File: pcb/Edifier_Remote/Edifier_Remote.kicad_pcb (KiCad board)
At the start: 2 copper layers, 4 parts, among them Q1 Q_NPN_BCE

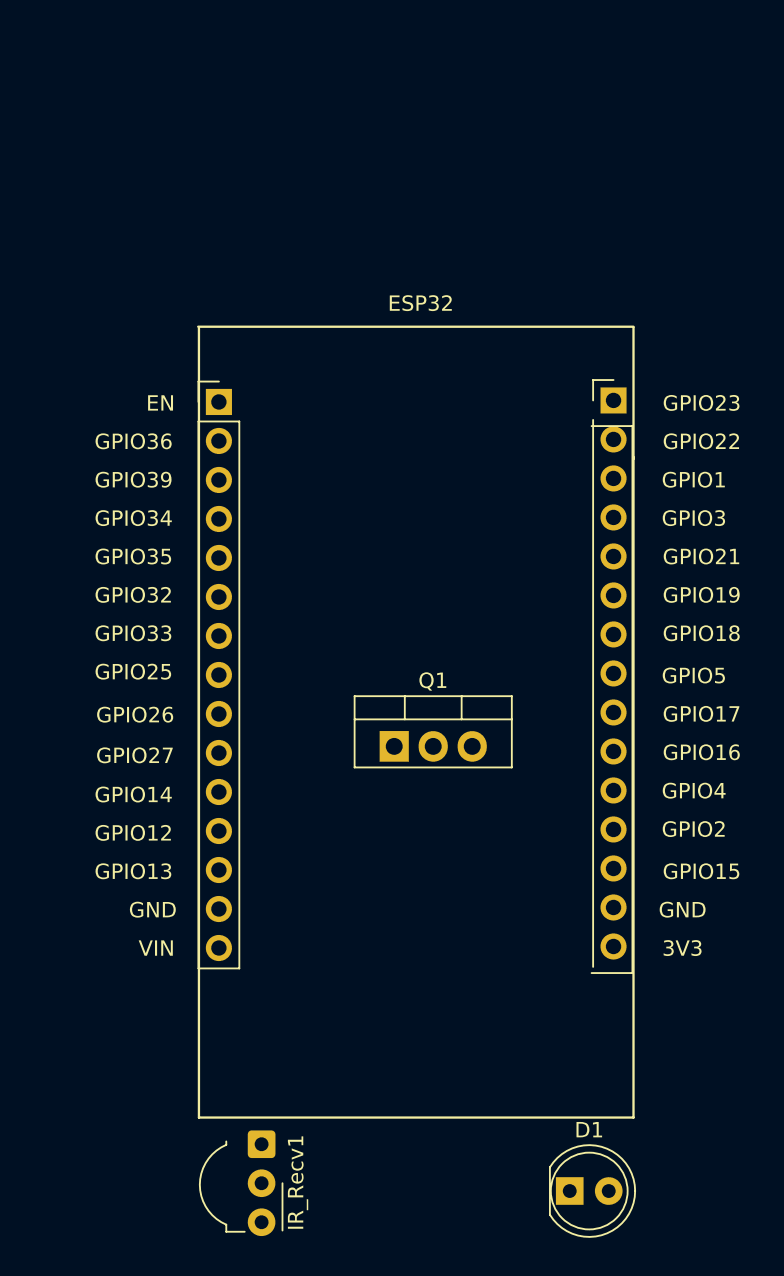
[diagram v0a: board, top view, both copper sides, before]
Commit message: finished board design
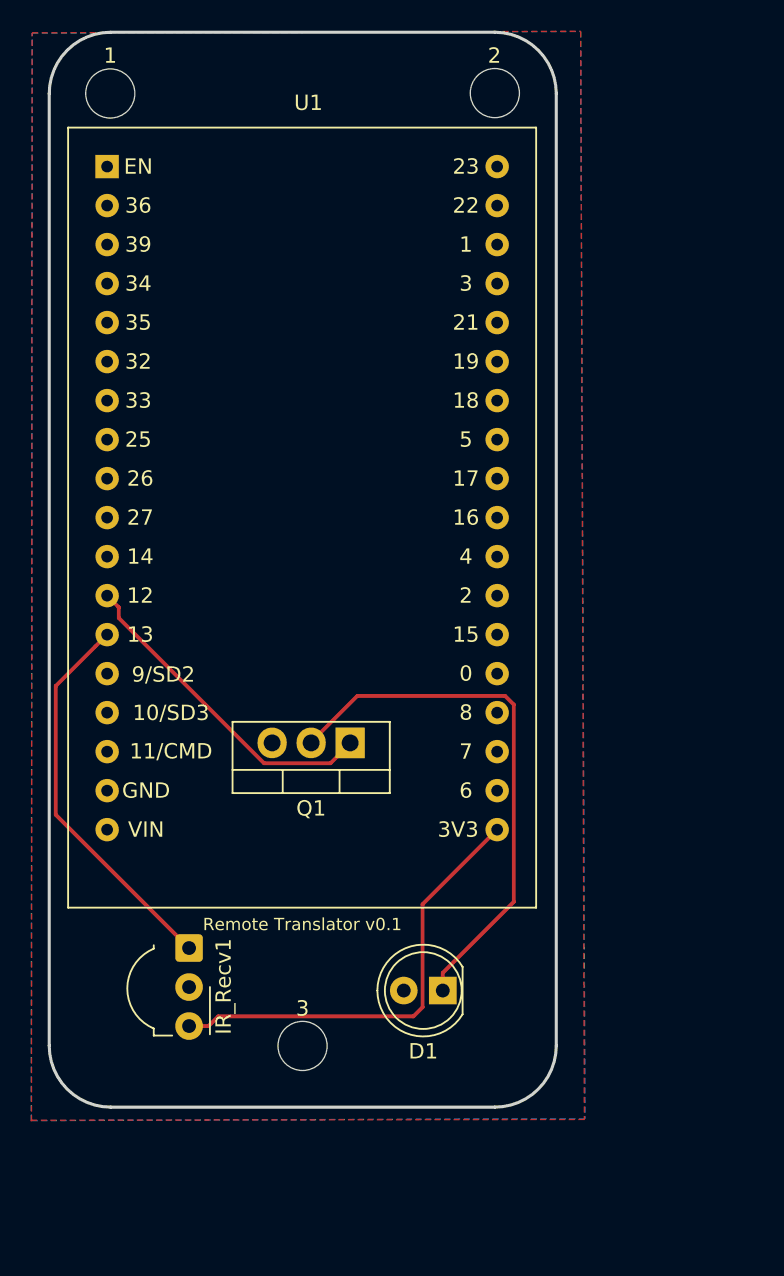
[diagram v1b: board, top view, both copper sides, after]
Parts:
- removed ESP32: ESP32_Devkit_DOIT_V1, ESP32:ESP32_Devkit_DOIT_V1
- added 1: MountingHole_3.2mm_M3, MountingHole:MountingHole_3.2mm_M3, F.Cu at (105.0, 70.3)
- added 2: MountingHole_3.2mm_M3, MountingHole:MountingHole_3.2mm_M3, F.Cu at (130.0, 70.2)
- added 3: MountingHole_3.2mm_M3, MountingHole:MountingHole_3.2mm_M3, F.Cu at (117.5, 132.3)
- added CUT: BoardCutout, ESP32:BoardCutout, F.Cu at (117.3, 98.3)
- added G***: LOGO, Logo:Logo, B.Cu at (117.0, 83.4)
- added U1: ESP32_DevKit, ESP32:ESP32_DevKit_36PIN, F.Cu at (114.9, 80.1)
- moved D1 15.5 mm to (126.6, 128.7), turned to 180 degrees
- moved IR_Recv1 13.6 mm to (110.1, 125.9)
- moved Q1 2.88 mm to (120.6, 112.5), turned to 180 degrees
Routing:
- net Net-(D1-Pad1): track 0.00 -> 35.3 mm
- net /3V3: track 0.00 -> 29.3 mm
- net /RECV: track 0.00 -> 25.4 mm
- net /SEND: track 0.00 -> 21.3 mm
- added copper zone on B.Cu, net /5V
- added copper zone on F.Cu, net GND
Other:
- board outline added: 33 x 70 mm
- board text added: "Remote Translator v0.1"
- board text added: "cristiansandu.ro"
